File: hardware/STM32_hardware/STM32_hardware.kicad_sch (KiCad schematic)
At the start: 23 parts, among them J1 Conn_02x07_Odd_Even, J2 Power, J3 Output, J4 Input, U1 STM32L021K4Tx, U2 MCP4801, U3 BU33SD5WG-TR

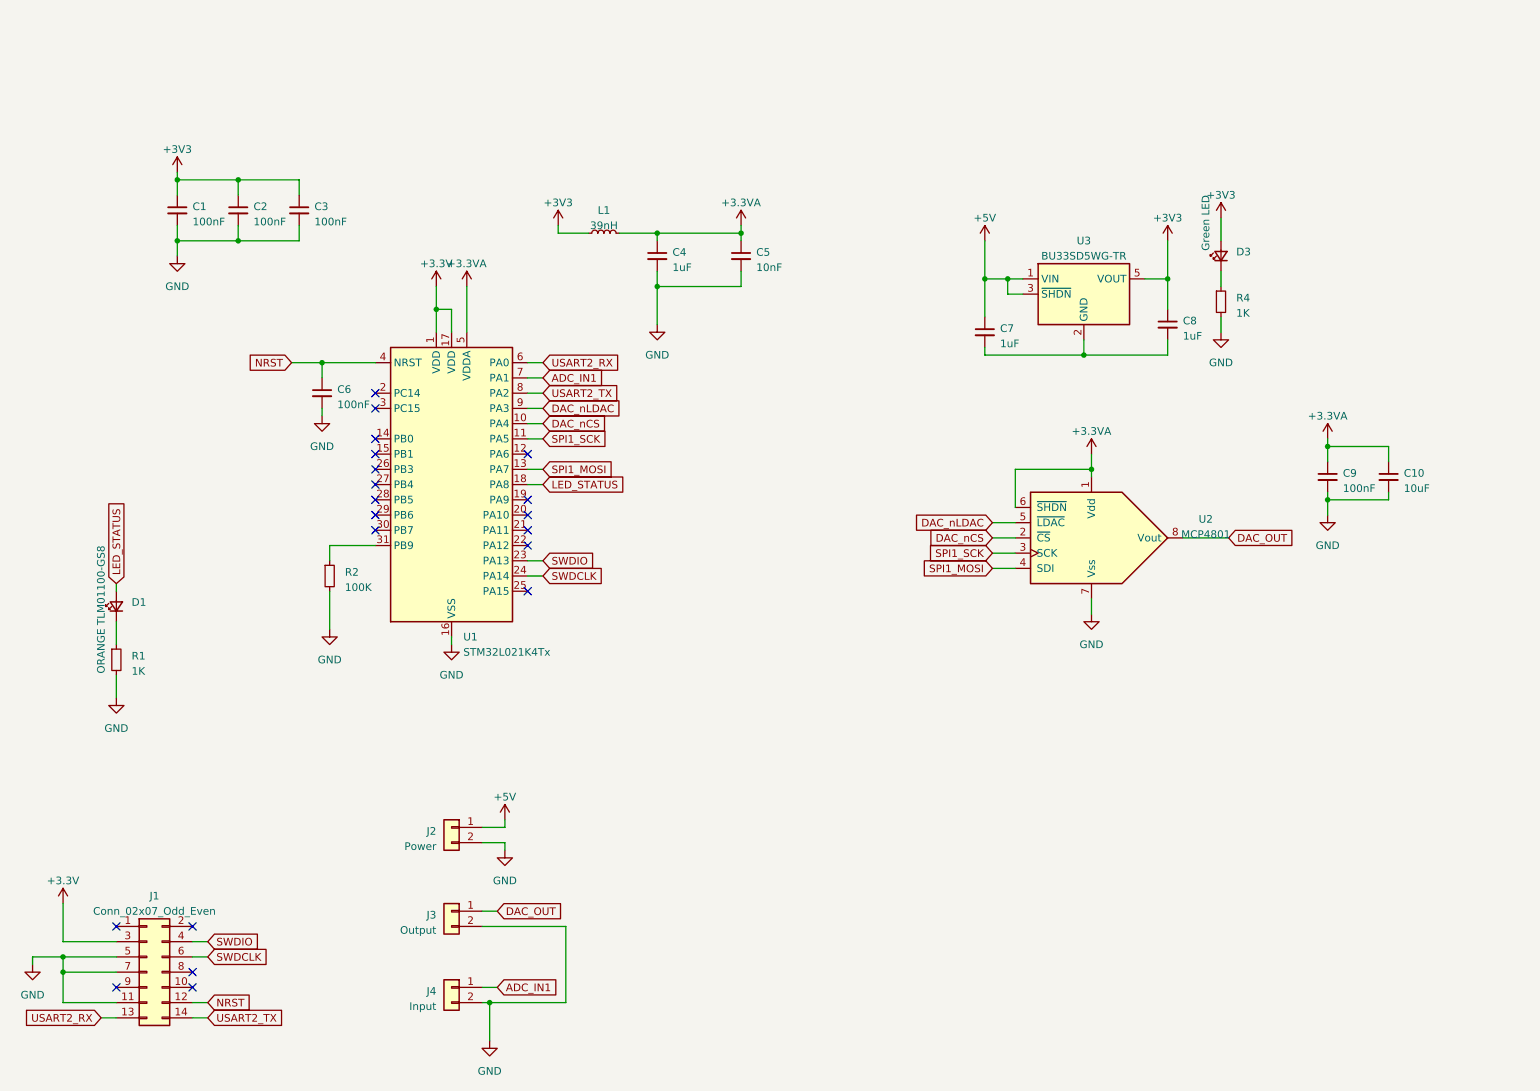
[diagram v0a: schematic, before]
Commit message: harware_PCB_contour
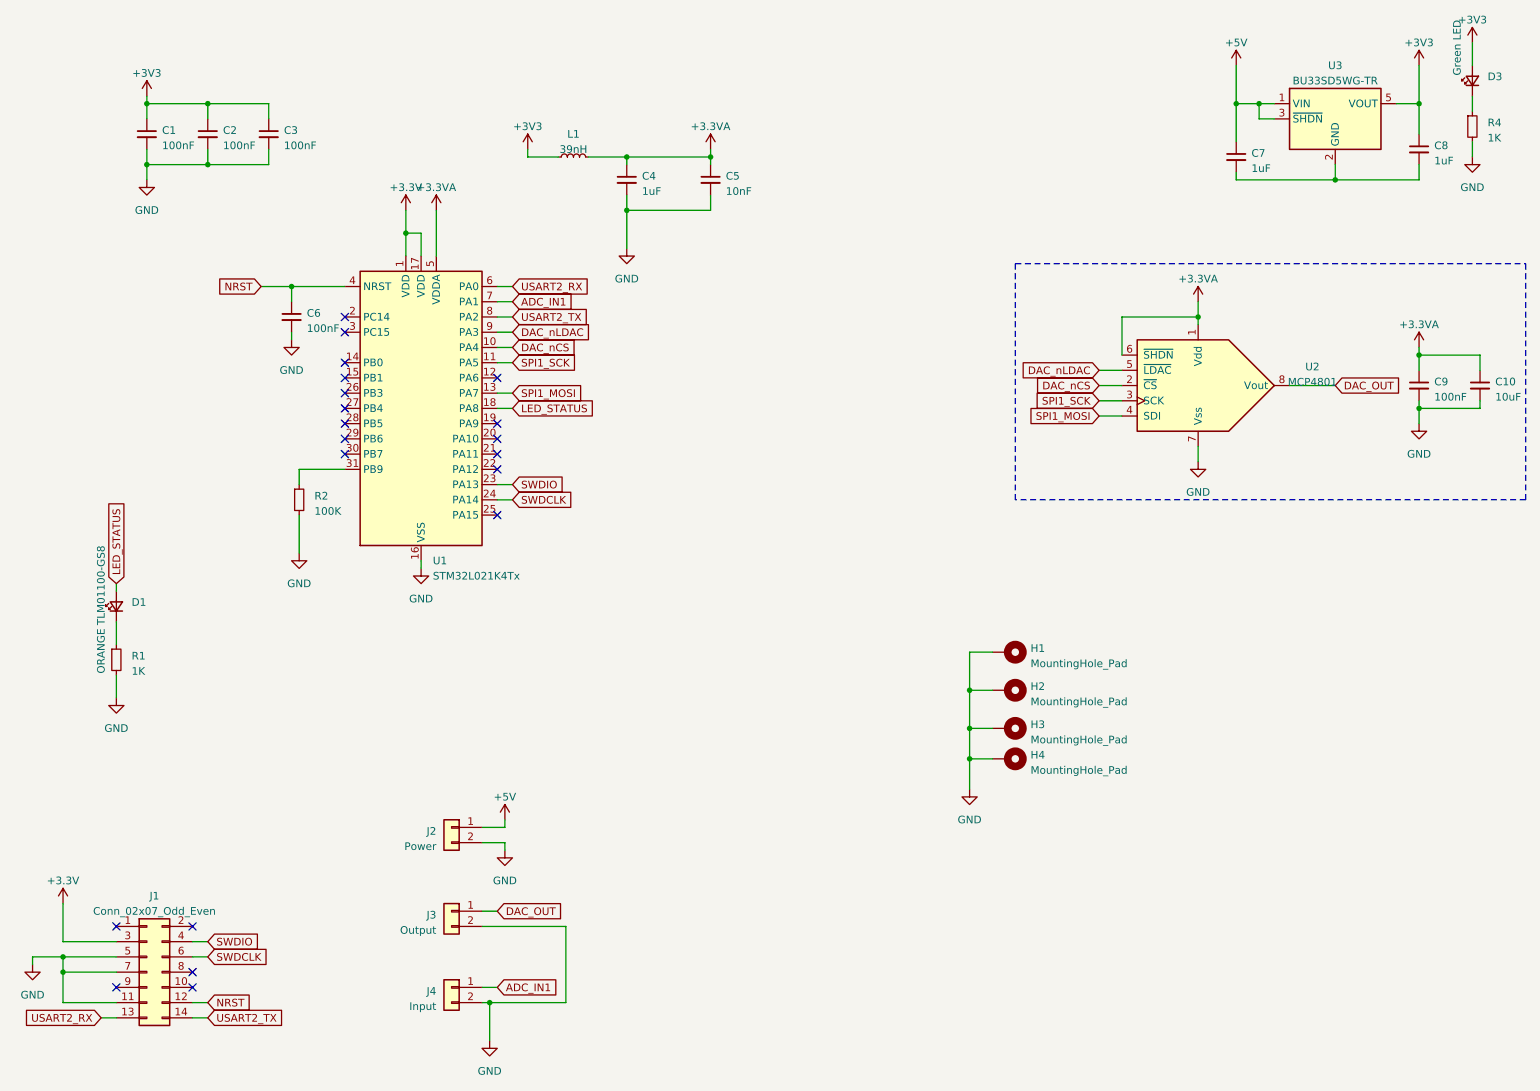
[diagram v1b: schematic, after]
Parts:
- added H1, H2, H3, H4: MountingHole_Pad, MountingHole:MountingHole_3.2mm_M3_Pad, symbol Mechanical:MountingHole_Pad
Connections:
- net GND: now also H1.1, H2.1, H3.1, H4.1
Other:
- moved on the sheet: C1, C10, C2, C3, C4, C5, C6, C7, C8, C9, D3, L1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
